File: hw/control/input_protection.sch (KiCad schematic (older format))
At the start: 6 parts, among them Q901 AOSP21357

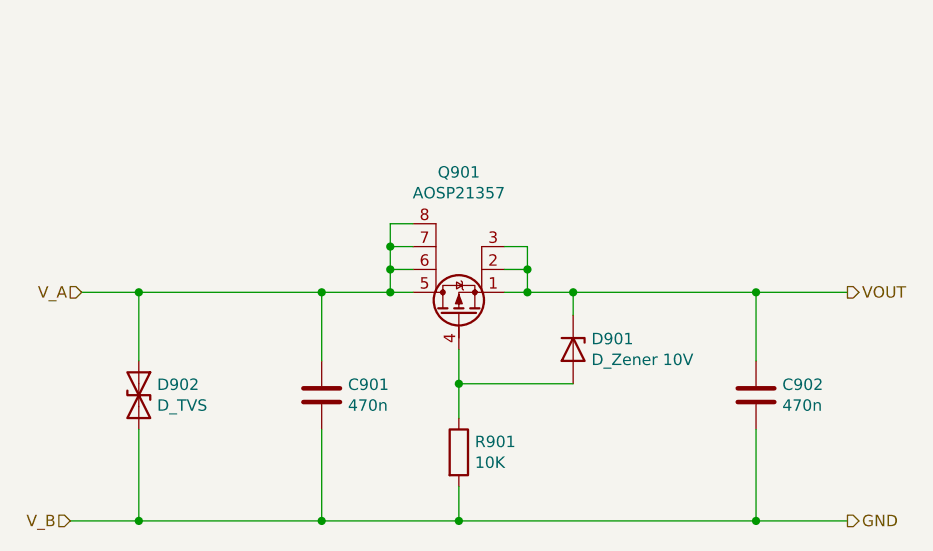
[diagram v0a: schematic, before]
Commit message: [hw] Incorporate suggestions
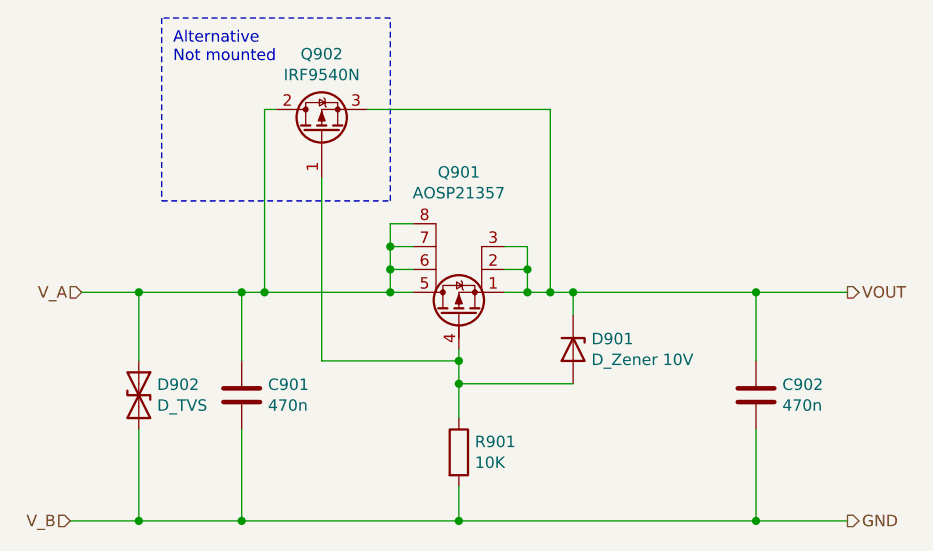
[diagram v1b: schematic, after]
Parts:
- added Q902: IRF9540N, Package_TO_SOT_THT:TO-220-3_Vertical, symbol Transistor_FET:IRF9540N
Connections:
- net VOUT: now also Q902.3 (S)
- net V_A: now also Q902.2 (D)
- net at D901.2 (A), Q901.4 (G), R901.1: now also Q902.1 (G)
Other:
- note added: "Alternative\nNot mounted"
- moved on the sheet: C901
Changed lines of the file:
@@
 Connection ~ 5450 3500
 Wire Wire Line
-	5450 3500 5650 3500
+	5450 3500 5550 3500
 Wire Wire Line
 	5450 3400 5450 3300
@@
 Connection ~ 5150 3900
 Wire Wire Line
-	5150 3900 5150 3750
+	5150 3900 5150 3800
 Wire Wire Line
 	5650 3600 5650 3500
@@
 Connection ~ 3750 3500
 Wire Wire Line
-	3750 3500 4550 3500
+	3750 3500 4200 3500
 Wire Wire Line
 	3750 4100 3750 4500
 Connection ~ 3750 4500
 Wire Wire Line
-	3750 4500 4550 4500
+	3750 4500 4200 4500
 Wire Wire Line
-	4550 3500 4550 3800
-Connection ~ 4550 3500
+	4200 3500 4200 3800
+Connection ~ 4200 3500
 Wire Wire Line
-	4550 3500 4850 3500
+	4200 3500 4300 3500
 Wire Wire Line
-	4550 4100 4550 4500
-Connection ~ 4550 4500
+	4200 4100 4200 4500
+Connection ~ 4200 4500
 Wire Wire Line
-	4550 4500 5150 4500
+	4200 4500 5150 4500
 $Comp
 L Device:D_TVS D902
@@
 L Device:C C901
 U 1 1 61464907
-P 4550 3950
-F 0 "C901" H 4665 3996 50  0000 L CNN
-F 1 "470n" H 4665 3905 50  0000 L CNN
-F 2 "Capacitor_SMD:C_0805_2012Metric_Pad1.18x1.45mm_HandSolder" H 4588 3800 50  0001 C CNN
-F 3 "~" H 4550 3950 50  0001 C CNN
-	1    4550 3950
+P 4200 3950
+F 0 "C901" H 4315 3996 50  0000 L CNN
+F 1 "470n" H 4315 3905 50  0000 L CNN
+F 2 "Capacitor_SMD:C_0805_2012Metric_Pad1.18x1.45mm_HandSolder" H 4238 3800 50  0001 C CNN
+F 3 "~" H 4200 3950 50  0001 C CNN
+	1    4200 3950
 	1    0    0    -1
 $EndComp
@@
 Wire Wire Line
 	6450 4500 6850 4500
+$Comp
+L Transistor_FET:IRF9540N Q902
+U 1 1 61697CC0
+P 4550 2800
+F 0 "Q902" V 4892 2800 50  0000 C CNN
+F 1 "IRF9540N" V 4801 2800 50  0000 C CNN
+F 2 "Package_TO_SOT_THT:TO-220-3_Vertical" H 4750 2725 50  0001 L CIN
+F 3 "http://www.irf.com/product-info/datasheets/data/irf9540n.pdf" H 4550 2800 50  0001 L CNN
+	1    4550 2800
+	0    -1   -1   0
+$EndComp
+Wire Wire Line
+	4550 3000 4550 3800
+Wire Wire Line
+	4550 3800 5150 3800
+Connection ~ 5150 3800
+Wire Wire Line
+	5150 3800 5150 3750
+Wire Wire Line
+	4350 2700 4300 2700
+Wire Wire Line
+	4300 2700 4300 3500
+Connection ~ 4300 3500
+Wire Wire Line
+	4300 3500 4850 3500
+Wire Wire Line
+	4750 2700 5550 2700
+Wire Wire Line
+	5550 2700 5550 3500
+Connection ~ 5550 3500
+Wire Wire Line
+	5550 3500 5650 3500
+Text Notes 3900 2500 0    50   ~ 0
+Alternative\nNot mounted
+Wire Notes Line
+	3850 3100 4850 3100
+Wire Notes Line
+	4850 3100 4850 2300
+Wire Notes Line
+	4850 2300 3850 2300
+Wire Notes Line
+	3850 2300 3850 3100
 $EndSCHEMATC
